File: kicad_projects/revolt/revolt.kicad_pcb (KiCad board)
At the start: 2 copper layers, 144.9 x 111.9 mm, 85 parts, among them J1 IDC-Header_2x07_P2.54mm_Verti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

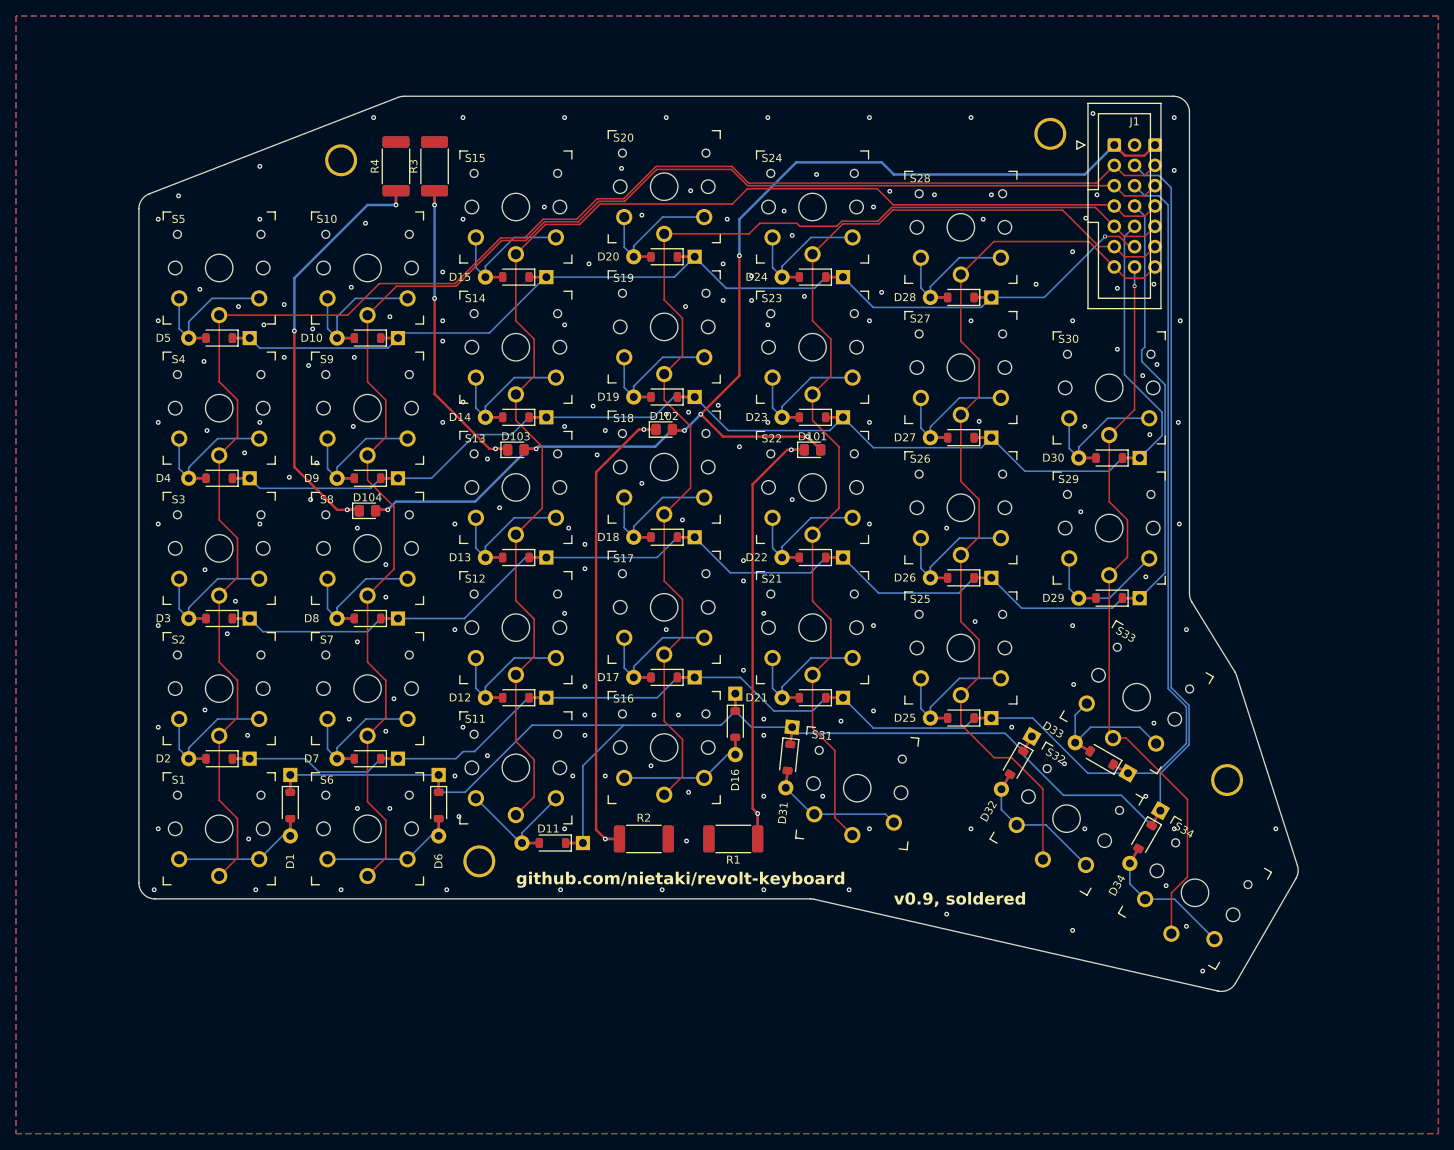
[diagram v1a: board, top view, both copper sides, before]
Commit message: Update to the latest files
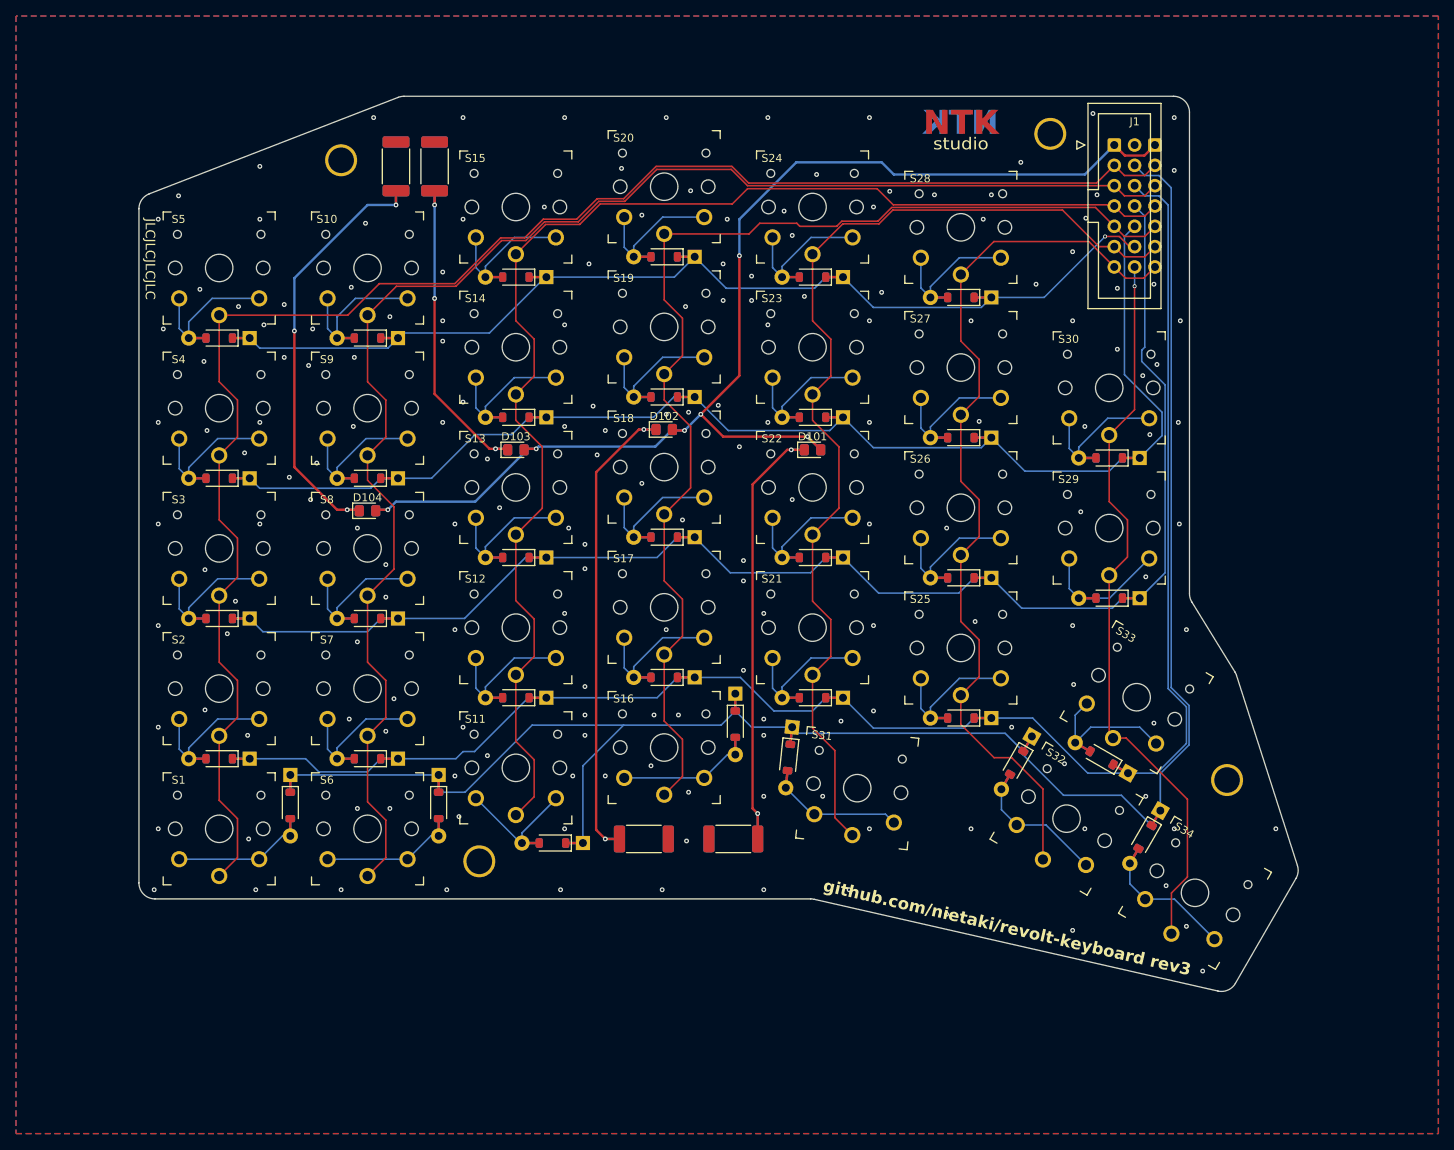
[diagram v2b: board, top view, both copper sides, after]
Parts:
- added REF**: NTK_studio, sdm:NTK_studio, F.Cu at (194.3, 64.9)
- added REF**: NTK_studio, sdm:NTK_studio, B.Cu at (194.3, 64.9)
- D1, D10, D11, D12, D13, D14, D15, D16, D17, D18, D19, D2, D20, D21, D22, D23, D24, D25, D26, D27, D28, D29, D3, D30, D31, D32, D33, D34, D4, D5, D6, D7, D8, D9, R1, R2, R3, R4: moved to B.Cu
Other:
- board text added: "JLCJLCJLCJLC"
- board text added: "github.com/nietaki/revolt-keyboard rev3"
- board text removed: "github.com/nietaki/revolt-keyboard"
- board text removed: "v0.9, soldered"
